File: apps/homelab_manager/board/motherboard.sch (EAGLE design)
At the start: 59 parts

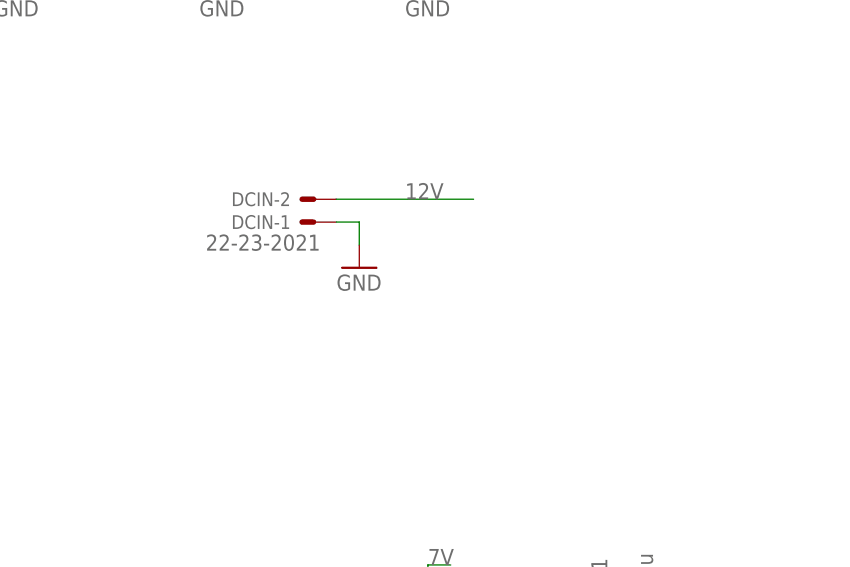
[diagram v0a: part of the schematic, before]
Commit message: Updated bazelisk + bazel
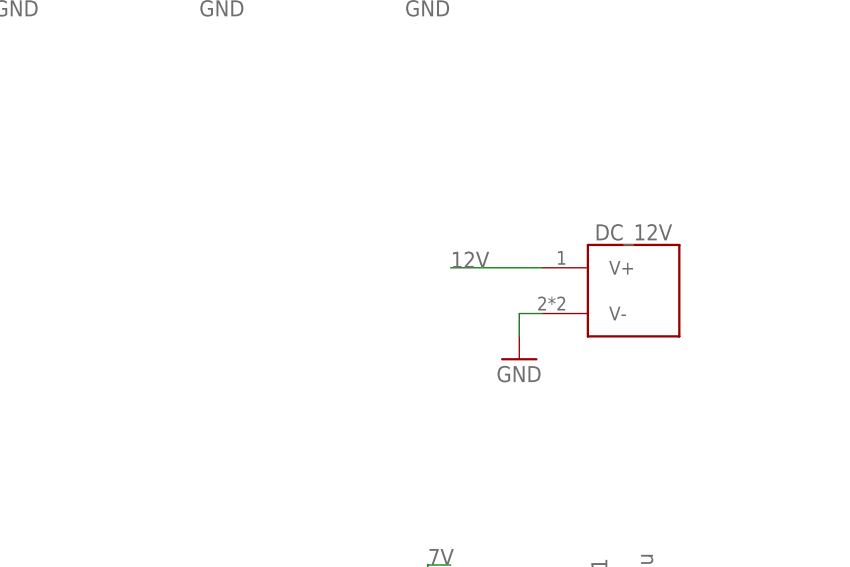
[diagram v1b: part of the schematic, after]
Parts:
- removed DCIN: 22-23-2021, con-molex:22-23-2021
- added DC_12V: DC_POWER_2.1MM, bzd:DC_POWER_2.1MM
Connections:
- net 12V: now also DC_12V.V+; no longer DCIN-2.S
- net GND: now also DC_12V.V-; no longer DCIN-1.S
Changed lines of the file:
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@@
 <parts>
 <part name="U$1" library="bzd" deviceset="ESP32_DEVKIT_V1" device=""/>
-<part name="DCIN" library="con-molex" library_urn="urn:adsk.eagle:library:165" deviceset="22-23-2021" device="" package3d_urn="urn:adsk.eagle:package:8078633/1"/>
-<part name="GND6" library="supply1" library_urn="urn:adsk.eagle:library:371" deviceset="GND" device=""/>
 <part name="U$4" library="bzd" deviceset="TPS561201" device=""/>
 <part name="GND12" library="supply1" library_urn="urn:adsk.eagle:library:371" deviceset="GND" device=""/>
@@
 <part name="D4" library="diode" library_urn="urn:adsk.eagle:library:210" deviceset="DIODE-" device="DO-214AC" package3d_urn="urn:adsk.eagle:package:43416/2" value="1N4148"/>
 <part name="RELAY" library="con-molex" library_urn="urn:adsk.eagle:library:165" deviceset="22-23-2021" device="" package3d_urn="urn:adsk.eagle:package:8078633/1"/>
+<part name="DC_12V" library="bzd" deviceset="DC_POWER_2.1MM" device=""/>
+<part name="GND22" library="supply1" library_urn="urn:adsk.eagle:library:371" deviceset="GND" device=""/>
 </parts>
 <sheets>
@@
 <attribute name="NAME" x="55.88" y="35.56" size="1.778" layer="95"/>
 </instance>
-<instance part="DCIN" gate="-1" x="-101.6" y="83.82" smashed="yes" rot="R180">
-<attribute name="NAME" x="-104.14" y="84.582" size="1.524" layer="95" rot="R180"/>
-<attribute name="VALUE" x="-100.838" y="82.423" size="1.778" layer="96" rot="R180"/>
-</instance>
-<instance part="DCIN" gate="-2" x="-101.6" y="86.36" smashed="yes" rot="R180">
-<attribute name="NAME" x="-104.14" y="87.122" size="1.524" layer="95" rot="R180"/>
-</instance>
-<instance part="GND6" gate="1" x="-96.52" y="78.74" smashed="yes">
-<attribute name="VALUE" x="-99.06" y="76.2" size="1.778" layer="96"/>
-</instance>
 <instance part="U$4" gate="G$1" x="-66.04" y="25.4" smashed="yes">
 <attribute name="NAME" x="-71.12" y="38.1" size="1.27" layer="95"/>
@@
 <instance part="RELAY" gate="-2" x="152.4" y="71.12" smashed="yes" rot="R180">
 <attribute name="NAME" x="149.86" y="71.882" size="1.524" layer="95" rot="R180"/>
+</instance>
+<instance part="DC_12V" gate="G$1" x="-68.58" y="76.2" smashed="yes">
+<attribute name="NAME" x="-70.358" y="81.788" size="1.778" layer="95"/>
+</instance>
+<instance part="GND22" gate="1" x="-78.74" y="68.58" smashed="yes">
+<attribute name="VALUE" x="-81.28" y="66.04" size="1.778" layer="96"/>
 </instance>
 </instances>
@@
 <nets>
 <net name="GND" class="0">
-<segment>
-<pinref part="DCIN" gate="-1" pin="S"/>
-<pinref part="GND6" gate="1" pin="GND"/>
-<wire x1="-99.06" y1="83.82" x2="-96.52" y2="83.82" width="0.1524" layer="91"/>
-<wire x1="-96.52" y1="83.82" x2="-96.52" y2="81.28" width="0.1524" layer="91"/>
-</segment>
 <segment>
 <pinref part="U$4" gate="G$1" pin="GND"/>
@@
 <wire x1="167.64" y1="48.26" x2="170.18" y2="48.26" width="0.1524" layer="91"/>
 <junction x="170.18" y="48.26"/>
+</segment>
+<segment>
+<pinref part="DC_12V" gate="G$1" pin="V-"/>
+<wire x1="-76.2" y1="73.66" x2="-78.74" y2="73.66" width="0.1524" layer="91"/>
+<pinref part="GND22" gate="1" pin="GND"/>
+<wire x1="-78.74" y1="73.66" x2="-78.74" y2="71.12" width="0.1524" layer="91"/>
 </segment>
 </net>
@@
 <net name="12V" class="0">
 <segment>
-<pinref part="DCIN" gate="-2" pin="S"/>
-<wire x1="-99.06" y1="86.36" x2="-83.82" y2="86.36" width="0.1524" layer="91"/>
-<label x="-91.44" y="86.36" size="1.778" layer="95"/>
-</segment>
-<segment>
 <pinref part="U$3" gate="G$1" pin="VIN+"/>
 <pinref part="R3" gate="G$1" pin="1"/>
@@
 <label x="-91.44" y="-53.34" size="1.778" layer="95"/>
 </segment>
+<segment>
+<pinref part="DC_12V" gate="G$1" pin="V+"/>
+<wire x1="-76.2" y1="78.74" x2="-86.36" y2="78.74" width="0.1524" layer="91"/>
+<label x="-86.36" y="78.74" size="1.778" layer="95"/>
+</segment>
 </net>
